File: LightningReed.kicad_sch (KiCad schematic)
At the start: 163 parts, among them P1 Conn_WallPlug, Q1 NCE65T180D, Q10 DMZ6005E, Q11 2N7002K, Q12 NCEP15T14D, Q13 BSS123, Q2 2N7002, Q3 1N60G, Q4 2N7002, Q5 2N7002K, Q6 2N7002K, Q7 NCE65T260K, Q8 NCE65T260K, Q9 NCE0102, T1 Transformer_2P_2S, U1 UCC28056, U2 78L05S, U3 LMC7111, U4 UCC28780, U5 UCC27712, U6 LM317G, U7 FODM8801A, U8 TL431DBZ, U9 UCC24612-1DBV

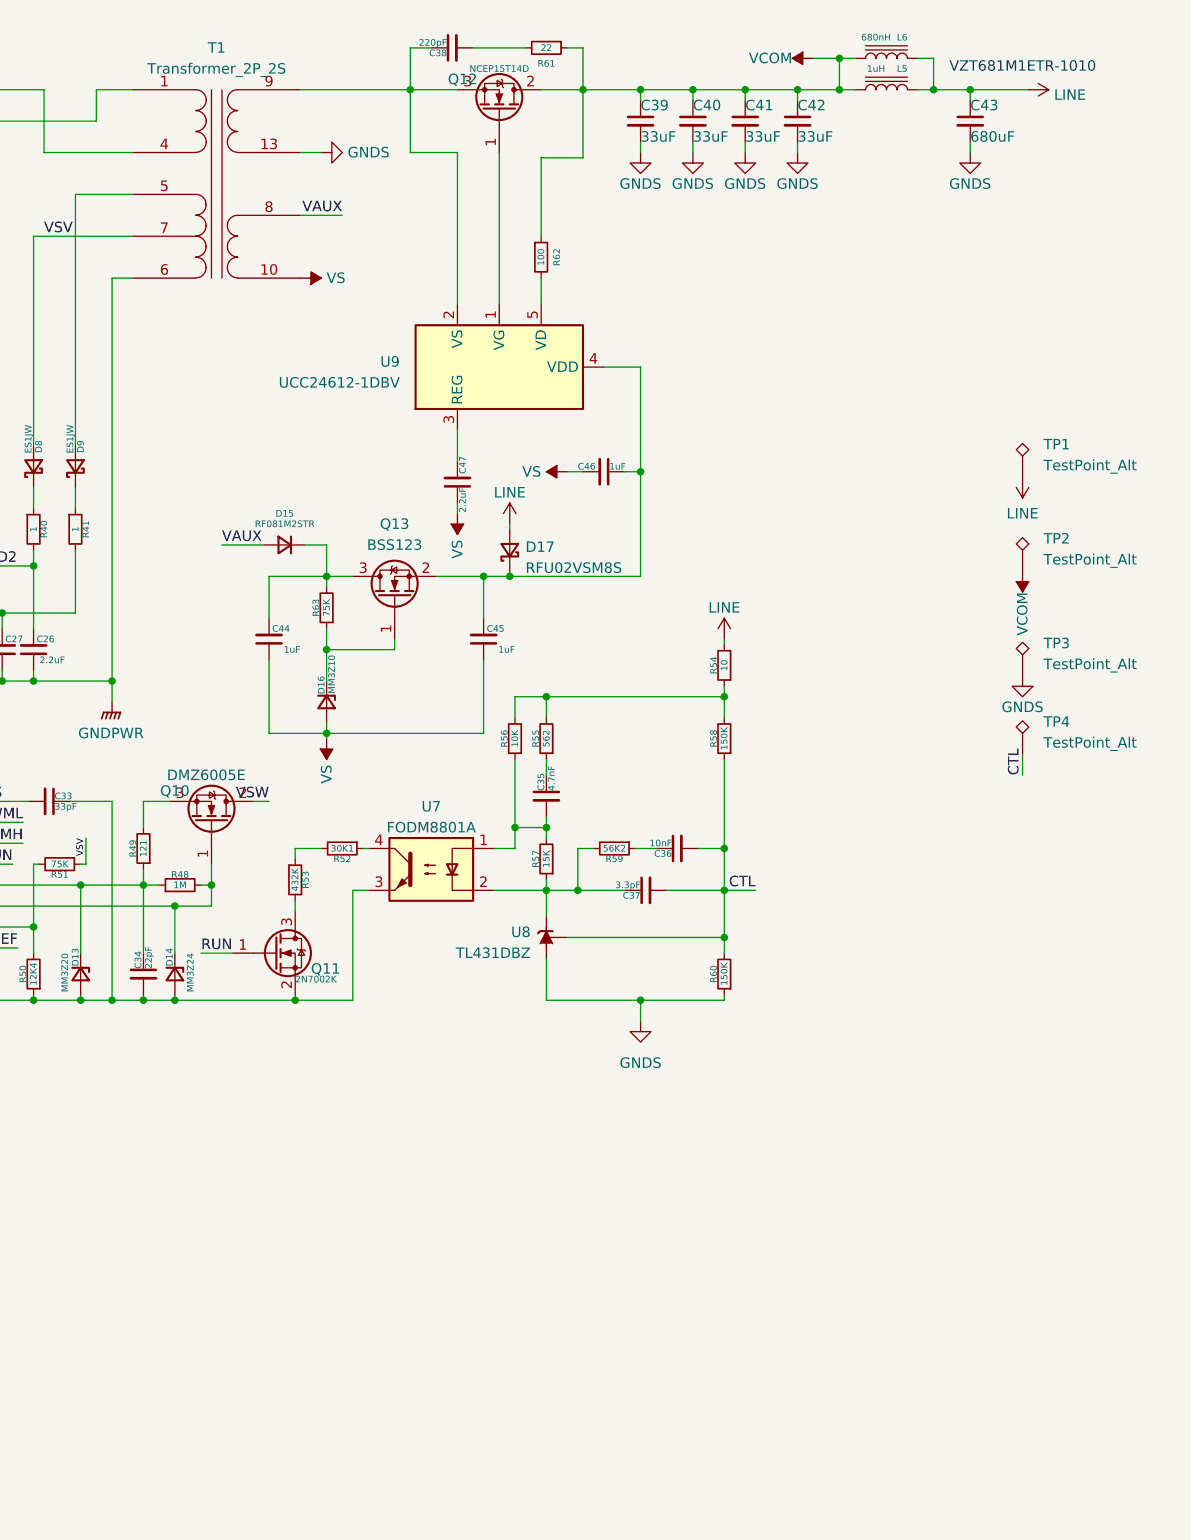
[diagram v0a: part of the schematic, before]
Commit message: SR layout
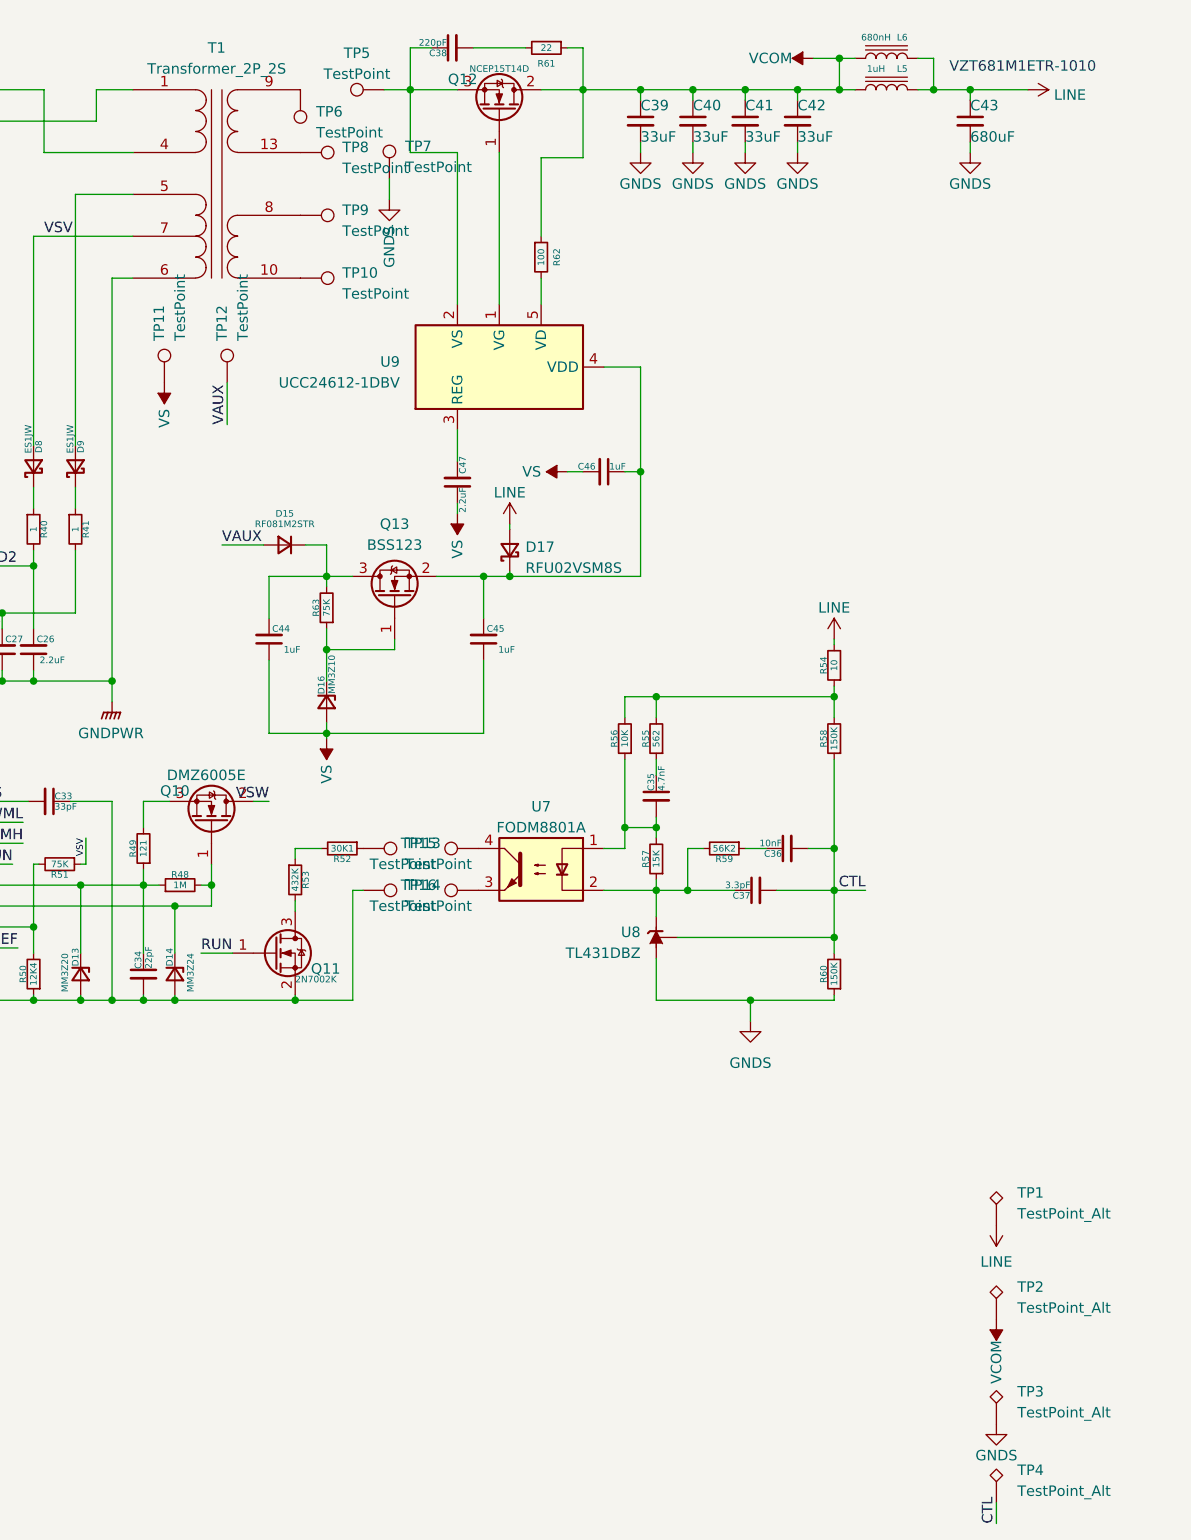
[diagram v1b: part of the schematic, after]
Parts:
- added TP10, TP11, TP12, TP13, TP14, TP15, TP16, TP9: TestPoint, Connector_Wire:SolderWire-0.15sqmm_1x01_D0.5mm_OD1.5mm, symbol Connector:TestPoint
- added TP5, TP6, TP7, TP8: TestPoint, Connector_Wire:SolderWire-1sqmm_1x01_D1.4mm_OD2.7mm, symbol Connector:TestPoint
- TP1: footprint Connector_Wire:SolderWire-0.5sqmm_1x01_D0.9mm_OD2.1mm -> Connector_Wire:SolderWire-1sqmm_1x01_D1.4mm_OD2.7mm
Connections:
- net GNDPWR: now also TP14.1; no longer U7.3
- net GNDS: now also TP7.1; no longer T1.13 (SB)
- net VAUX: now also TP12.1; no longer T1.8 (SC)
- net VS: now also TP11.1; no longer T1.10 (SD)
- net at R52.1: now also TP13.1; no longer U7.4
- net at C38.1, Q12.3 (S), U9.2 (VS): now also TP5.1; no longer T1.9 (SA)
- new net: TP16.1, U7.3
- new net: T1.9 (SA), TP6.1
- new net: T1.10 (SD), TP10.1
- new net: T1.13 (SB), TP8.1
- new net: T1.8 (SC), TP9.1
- new net: TP15.1, U7.4
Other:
- moved on the sheet: C35, C36, C37, R54, R55, R56, R57, R58, R59, R60, TP1, TP2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
